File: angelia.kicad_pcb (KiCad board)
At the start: 2 copper layers, 160 x 120 mm, 206 parts, among them J10 Conn_Coaxial, J15 Conn_02x05_Top_Bottom, J16 Conn_02x13_Top_Bottom, J18 Conn_02x05_Top_Bottom, J25 Conn_Coaxial, J3 Conn_Coaxial, J5 Conn_Coaxial, P1 Conn_02x05_Top_Bottom, P2 Conn_02x05_Top_Bottom, U10 LTC2208xUP, U18 LTC2208xUP, U5 EP4CE115F780

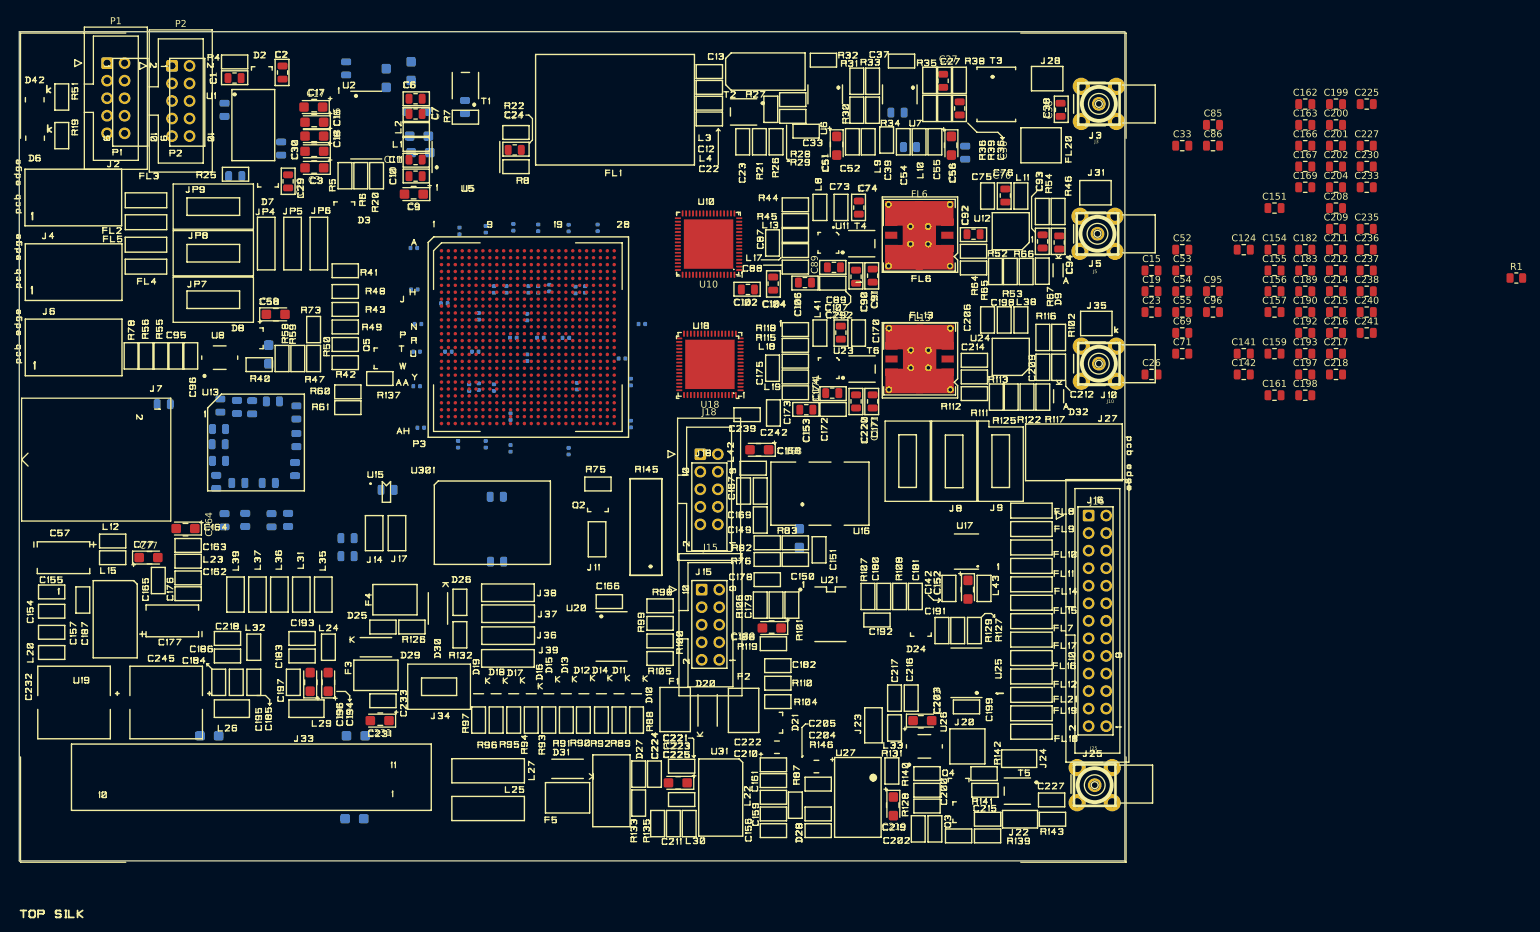
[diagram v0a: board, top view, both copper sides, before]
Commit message: all decoupling done
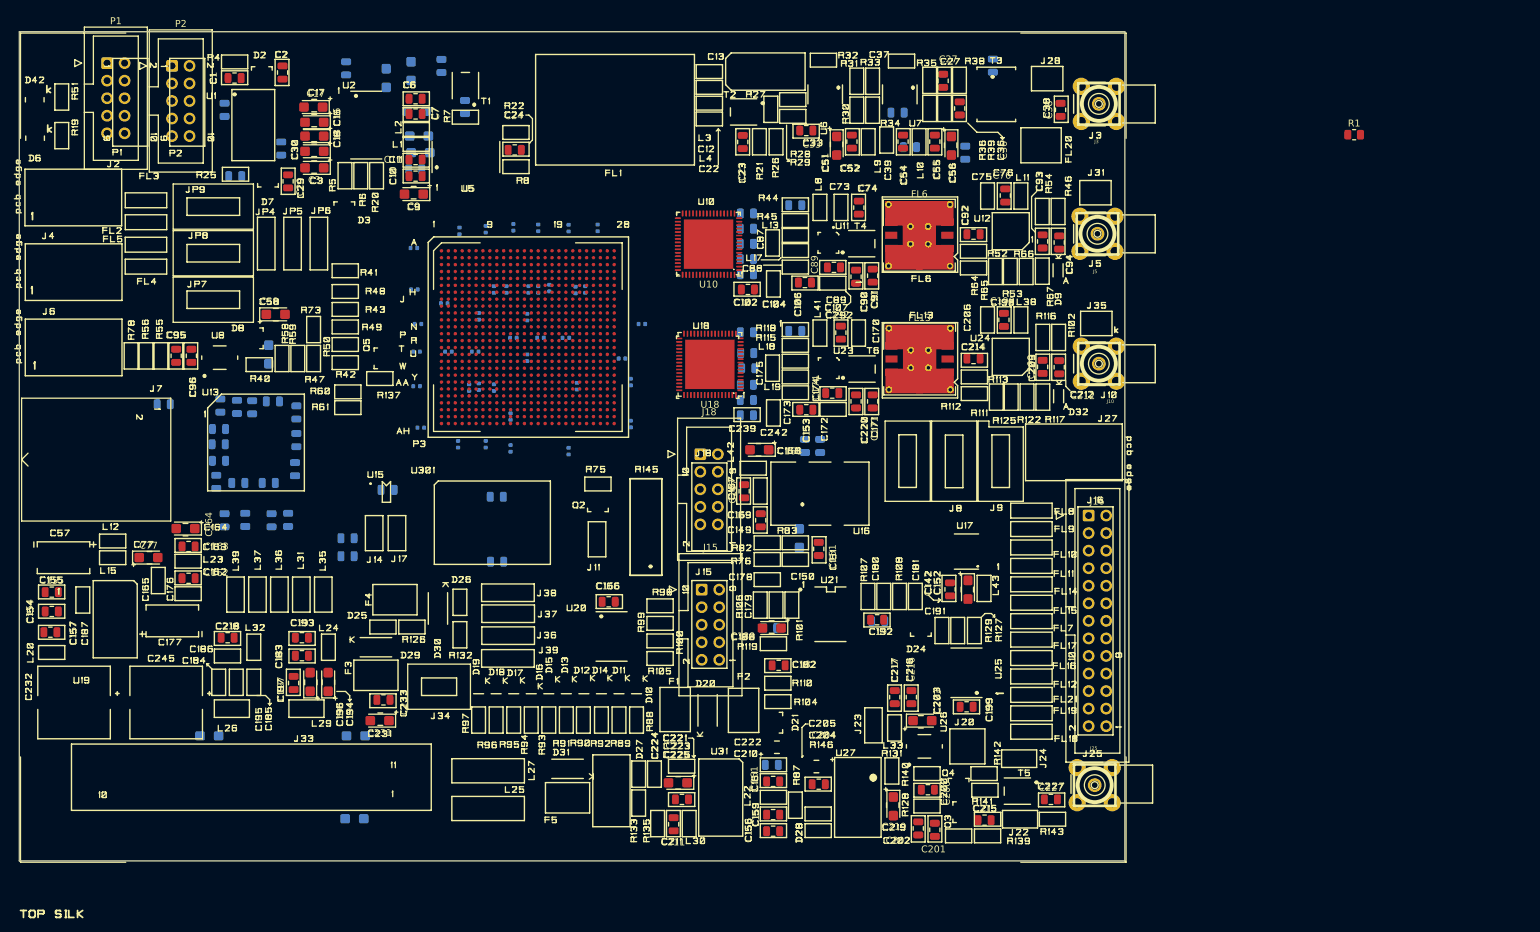
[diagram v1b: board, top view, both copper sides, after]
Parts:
- C104, C124, C141, C15, C189, C19, C190, C208, C230, C235, C236, C237, C238, C240, C241, C26, C53, C69, C71, C85, C86: moved to B.Cu
- moved C154 184.5 mm to (68.2, 118.4)
- moved C157 183.1 mm to (68.0, 121.4)
- moved C155 183.0 mm to (68.2, 115.6)
- moved C162 175.6 mm to (88.0, 113.6)
- moved C163 172.7 mm to (88.0, 109.0)
- moved C218 164.9 mm to (93.7, 122.2)
- moved C233 160.5 mm to (116.2, 131.2)
- moved C183 155.5 mm to (104.4, 124.8)
- moved C197 153.1 mm to (103.2, 128.8), turned to 90 degrees
- moved C193 150.9 mm to (104.4, 122.2)
- moved C95 150.4 mm to (86.2, 81.4), turned to 90 degrees
- moved C96 148.0 mm to (88.4, 81.4), turned to 90 degrees
- moved C225 141.2 mm to (159.4, 145.6)
- moved C211 126.9 mm to (158.2, 149.2), turned to 90 degrees
- moved C230 122.1 mm to (172.4, 140.6), turned to 180 degrees
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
